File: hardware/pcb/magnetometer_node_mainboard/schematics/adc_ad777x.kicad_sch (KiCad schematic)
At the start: 1 part, among them U8 AD7779

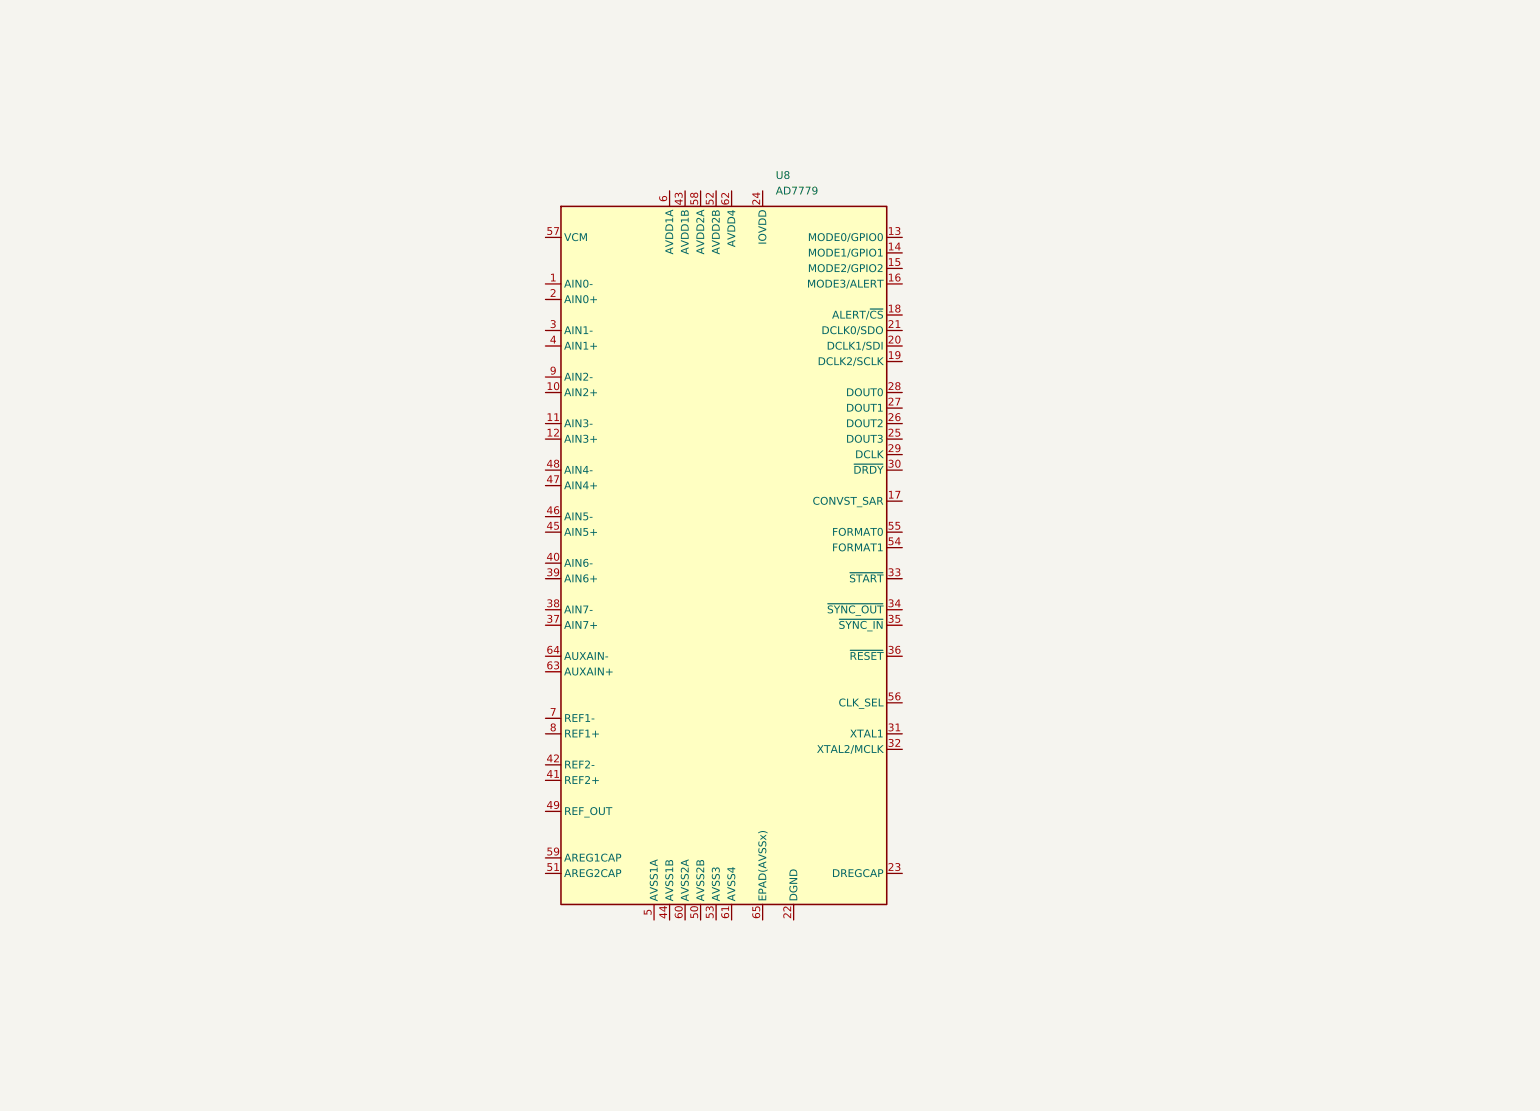
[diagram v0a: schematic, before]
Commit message: first code for the v1
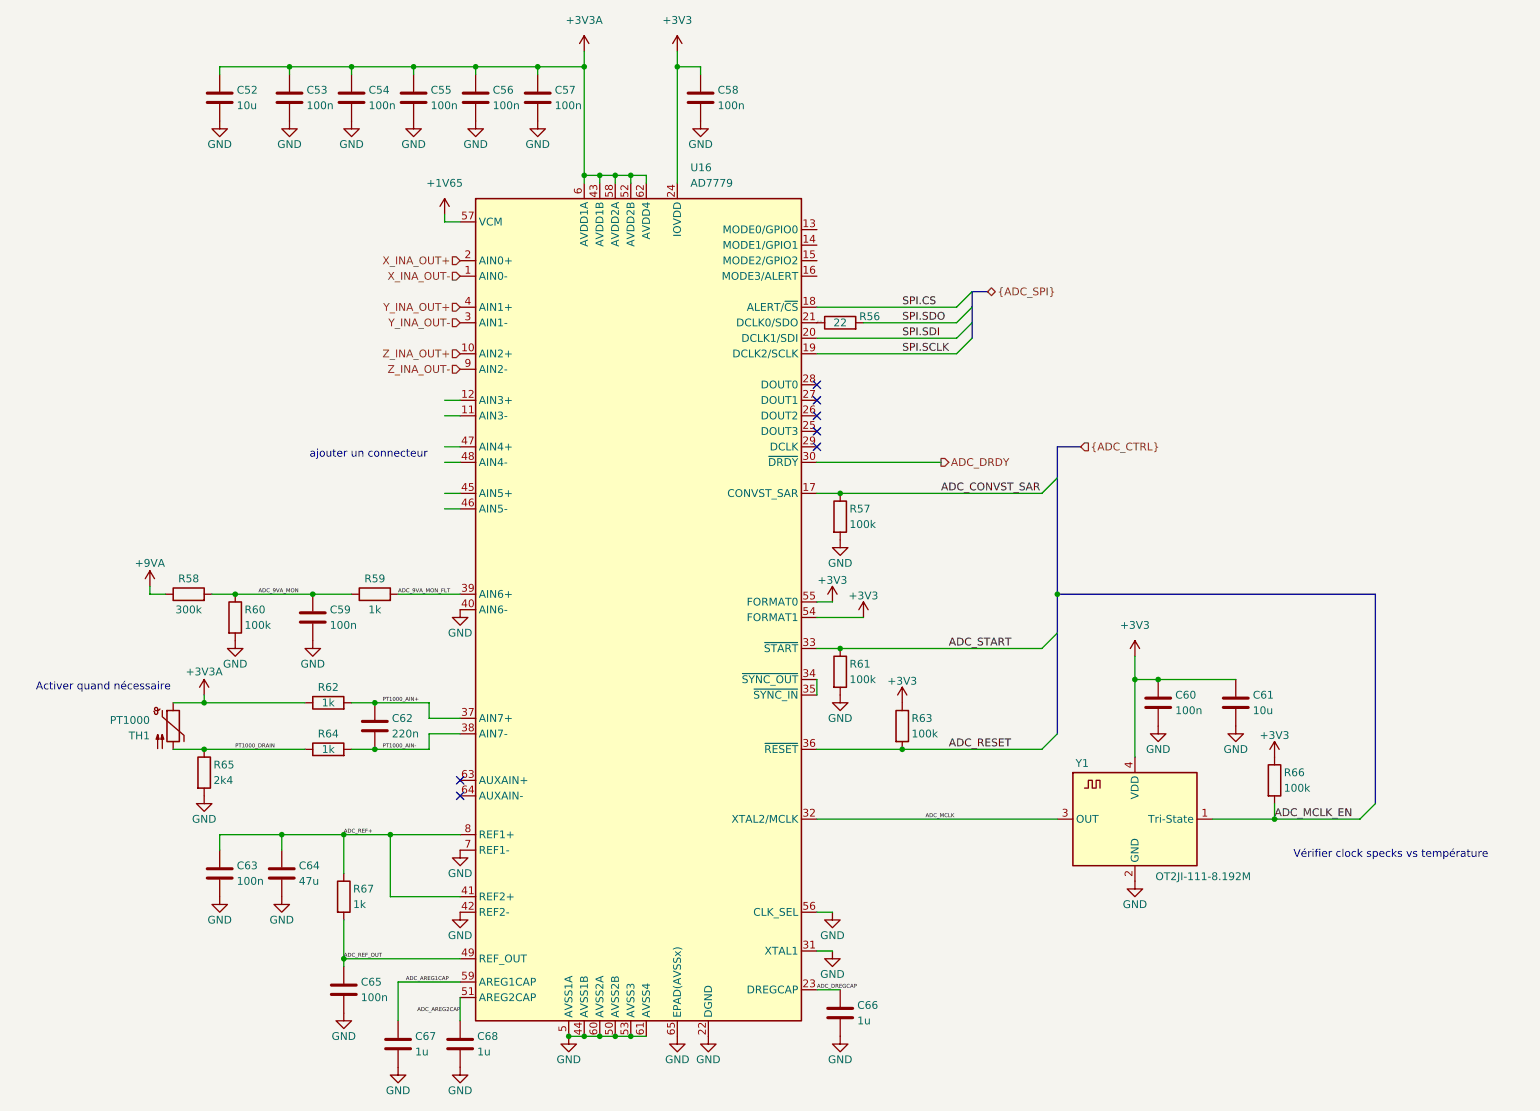
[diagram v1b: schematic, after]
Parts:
- removed U8: AD7779, Package_DFN_QFN:QFN-64-1EP_9x9mm_P0.5mm_EP7.65x7.65mm, symbol Analog_ADC:AD7779
- added C52, C61: 10u, Capacitor_SMD:C_0805_2012Metric, symbol Device:C
- added C53, C54, C55, C56, C57, C58, C59, C60, C63, C65: 100n, Capacitor_SMD:C_0603_1608Metric, symbol Device:C
- added C62: 220n, Capacitor_SMD:C_0603_1608Metric, symbol Device:C
- added C64: 47u, Capacitor_SMD:C_1206_3216Metric, symbol Device:C
- added C66, C67, C68: 1u, Capacitor_SMD:C_0805_2012Metric, symbol Device:C
- added R56: 22, Resistor_SMD:R_0603_1608Metric, symbol Device:R
- added R57, R60, R61, R63, R66: 100k, Resistor_SMD:R_0603_1608Metric, symbol Device:R
- added R58: 300k, Resistor_SMD:R_0603_1608Metric, symbol Device:R
- added R59, R62, R64, R67: 1k, Resistor_SMD:R_0603_1608Metric, symbol Device:R
- added R65: 2k4, Resistor_SMD:R_0805_2012Metric, symbol Device:R
- added TH1: PT1000, symbol Sensor_Temperature:PT1000
- added U16: AD7779, Package_DFN_QFN:QFN-64-1EP_9x9mm_P0.5mm_EP7.65x7.65mm, symbol magnode_symbols:AD7779_custom
- added Y1: OT2JI-111-8.192M, Crystal:Crystal_SMD_3225-4Pin_3.2x2.5mm, symbol magnode_symbols:YSO110TR
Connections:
- new net: U16.34 (~{SYNC_OUT}), U16.35 (~{SYNC_IN})
- new net +1V65: U16.57 (VCM)
- new net +3V3: C58.1, C60.1, C61.1, R63.1, R66.1, U16.24 (IOVDD), U16.54 (FORMAT1), U16.55 (FORMAT0), Y1.4 (VDD)
- new net +3V3A: C52.1, C53.1, C54.1, C55.1, C56.1, C57.1, R62.1, TH1.1, U16.43 (AVDD1B), U16.52 (AVDD2B), U16.58 (AVDD2A), U16.6 (AVDD1A), U16.62 (AVDD4)
- new net +9VA: R58.1
- new net ADC_9VA_MON: C59.1, R58.2, R59.1, R60.1
- new net ADC_9VA_MON_FLT: R59.2, U16.39 (AIN6+)
- new net ADC_AREG1CAP: C67.1, U16.59 (AREG1CAP)
- new net ADC_AREG2CAP: C68.1, U16.51 (AREG2CAP)
- new net ADC_CONVST_SAR: R57.1, U16.17 (CONVST_SAR)
- new net ADC_DRDY: U16.30 (~{DRDY})
- new net ADC_DREGCAP: C66.1, U16.23 (DREGCAP)
- new net ADC_MCLK: U16.32 (XTAL2/MCLK), Y1.3 (OUT)
- new net ADC_MCLK_EN: R66.2, Y1.1 (Tri-State)
- new net ADC_REF+: C63.1, C64.1, R67.1, U16.41 (REF2+), U16.8 (REF1+)
- new net ADC_REF_OUT: C65.1, R67.2, U16.49 (REF_OUT)
- new net ADC_RESET: R63.2, U16.36 (~{RESET})
- new net ADC_SDO: R56.1, U16.21 (DCLK0/SDO)
- new net ADC_START: R61.1, U16.33 (~{START})
- new net GND: C52.2, C53.2, C54.2, C55.2, C56.2, C57.2, C58.2, C59.2, C60.2, C61.2, C63.2, C64.2, C65.2, C66.2, C67.2, C68.2, R57.2, R60.2, R61.2, R65.2, U16.22 (DGND), U16.31 (XTAL1), U16.40 (AIN6-), U16.42 (REF2-), U16.44 (AVSS1B), U16.5 (AVSS1A), U16.50 (AVSS2B), U16.53 (AVSS3), U16.56 (CLK_SEL), U16.60 (AVSS2A), U16.61 (AVSS4), U16.65 (EPAD(AVSSx)), U16.7 (REF1-), Y1.2 (GND)
- new net PT1000_AIN+: C62.1, R62.2, U16.37 (AIN7+)
- new net PT1000_AIN-: C62.2, R64.2, U16.38 (AIN7-)
- new net PT1000_DRAIN: R64.1, R65.1, TH1.2
- new net SPI.CS: U16.18 (ALERT/~{CS})
- new net SPI.SCLK: U16.19 (DCLK2/SCLK)
- new net SPI.SDI: U16.20 (DCLK1/SDI)
- new net SPI.SDO: R56.2
- new net X_INA_OUT+: U16.2 (AIN0+)
- new net X_INA_OUT-: U16.1 (AIN0-)
- new net Y_INA_OUT+: U16.4 (AIN1+)
- new net Y_INA_OUT-: U16.3 (AIN1-)
- new net Z_INA_OUT+: U16.10 (AIN2+)
- new net Z_INA_OUT-: U16.9 (AIN2-)
- no-connect marks 0 -> 7
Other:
- note added: "Activer quand nécessaire"
- note added: "Vérifier clock specks vs température"
- note added: "ajouter un connecteur"
